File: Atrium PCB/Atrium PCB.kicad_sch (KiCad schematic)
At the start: 495 parts, among them J1 Conn_01x05_Pin, SW1 EC11E09244BS, SW10 SW_Push, SW11 SW_Push, SW13 SW_Push, SW14 SW_Push, SW15 SW_Push, SW16 SW_Push, SW18 SW_Push, SW19 SW_Push, SW2 SKRPACE010, SW20 SW_Push, SW22 SW_Push, SW23 SW_Push, SW24 SW_Push, SW26 SW_Push, SW27 SW_Push, SW28 SW_Push, SW3 SKRPACE010, SW30 SW_Push, SW31 SW_Push, SW32 SW_Push, SW34 SW_Push, SW35 SW_Push, SW36 SW_Push, SW38 SW_Push, SW39 SW_Push, SW4 SW_Push, SW40 SW_Push, SW42 SW_Push, SW43 SW_Push, SW44 SW_Push, SW45 SW_Push, SW46 SW_Push, SW47 SW_Push, SW48 SW_Push, SW49 SW_Push, SW5 SW_Push, SW50 SW_Push, SW51 SW_Push, SW52 SW_Push, SW53 SW_Push, SW54 SW_Push, SW6 SW_Push, SW8 SW_Push, SW9 SW_Push, U12 AP2112K-3.3, U2 LSM6DS3TR-C, U6 SN74LVC1T45DBVR, X1 X322512MSB4SI

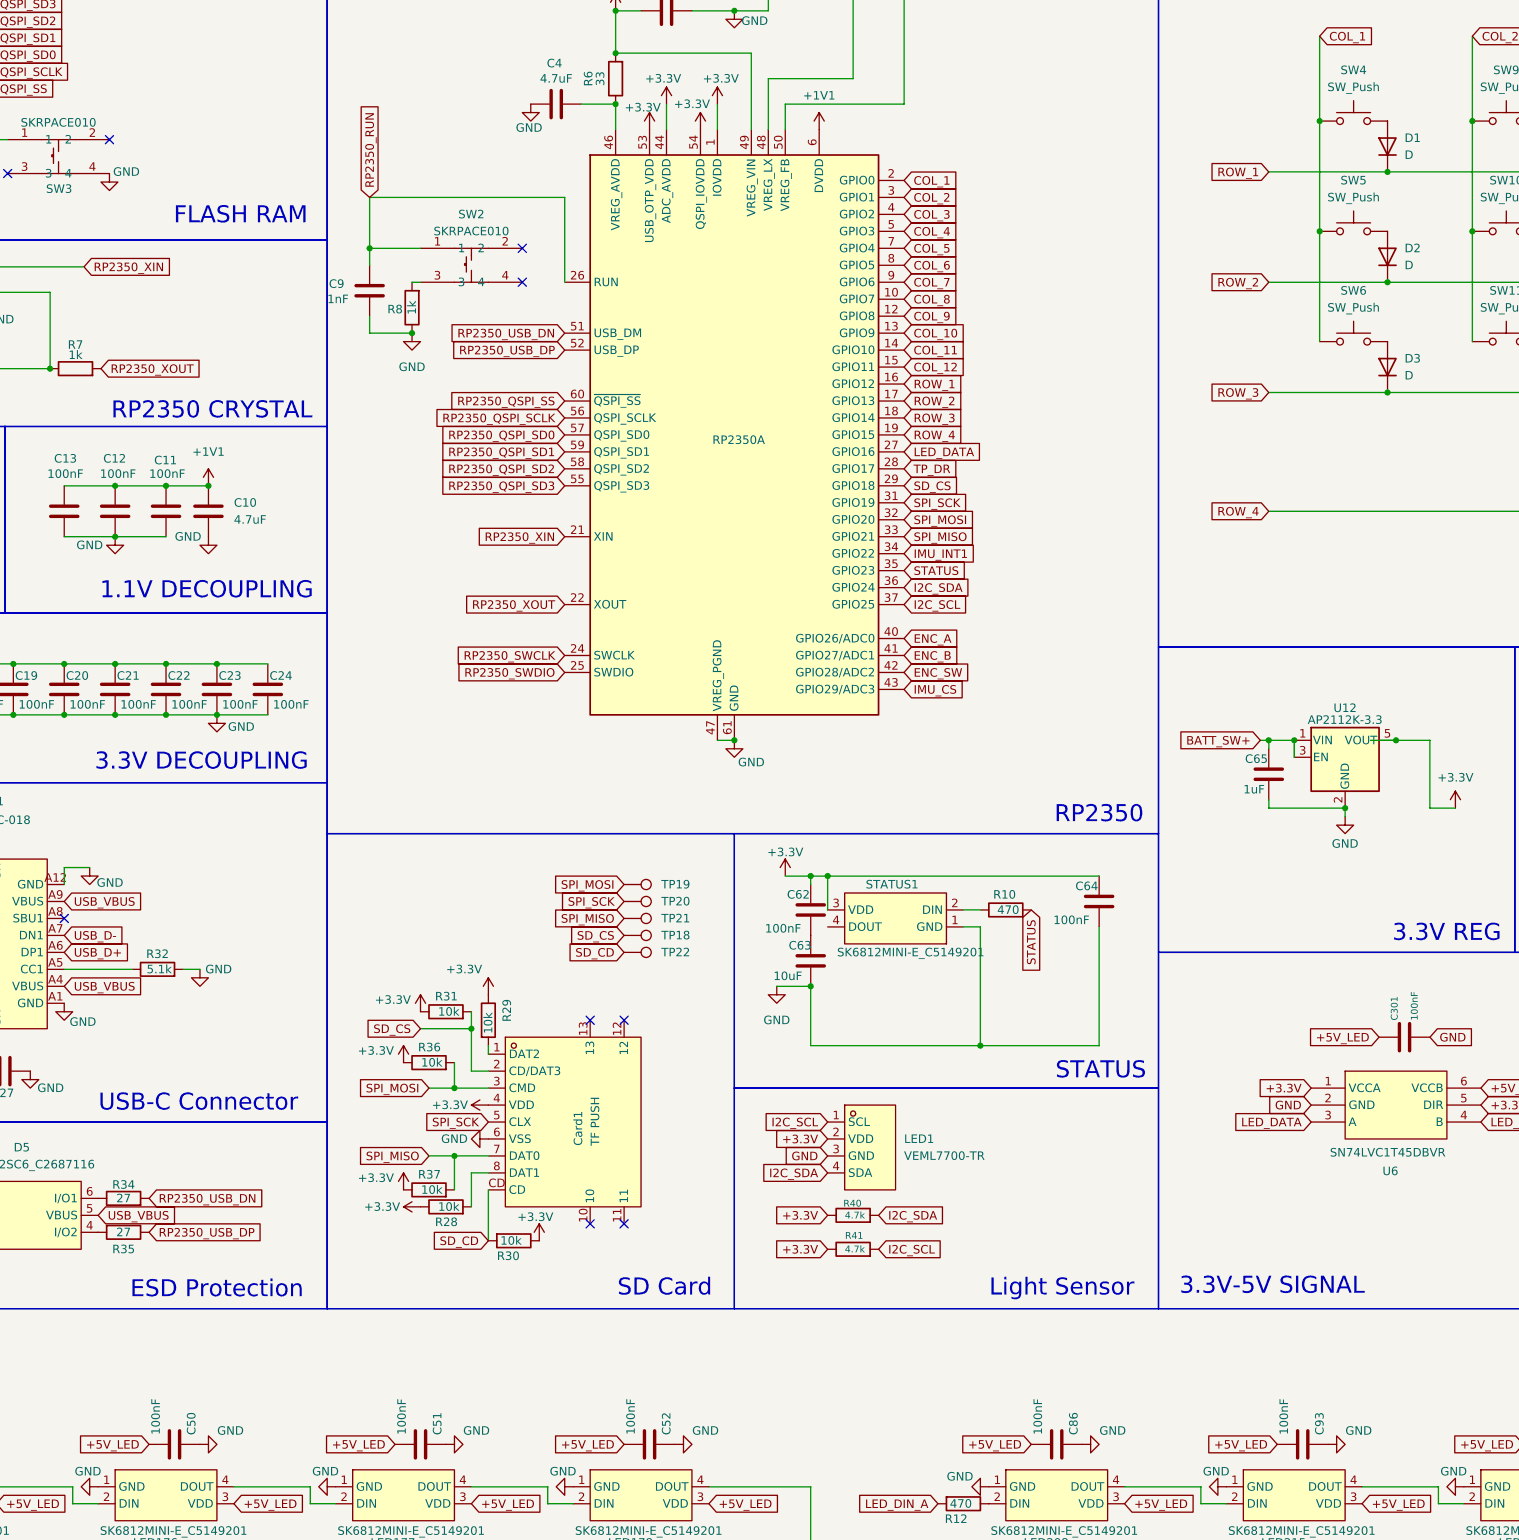
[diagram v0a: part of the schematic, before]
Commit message: sync
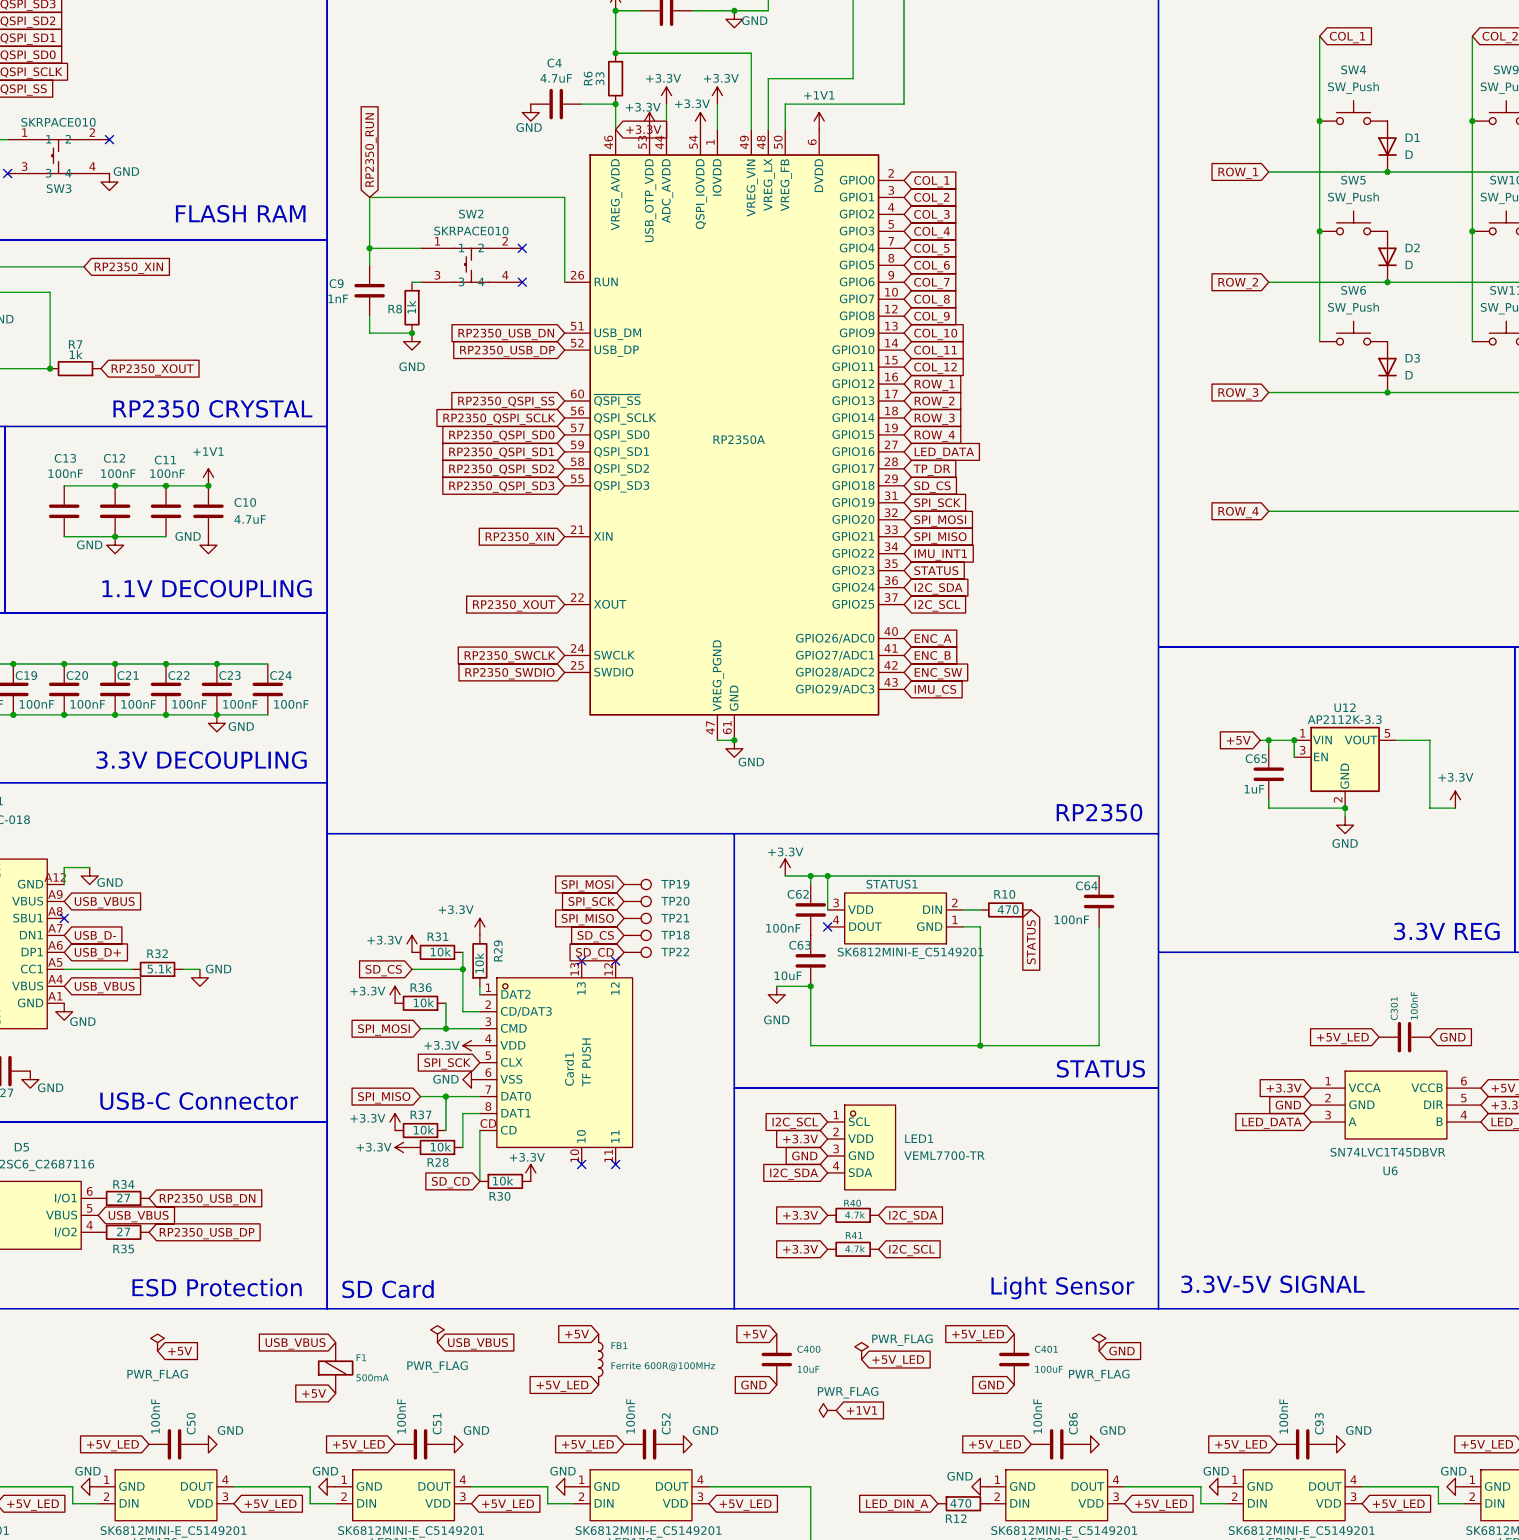
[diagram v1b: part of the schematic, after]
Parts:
- added C400: 10uF, Capacitor_SMD:C_0805_2012Metric, symbol Device:C
- added C401: 100uF, Capacitor_SMD:C_1206_3216Metric, symbol Device:C
- added F1: 500mA, Fuse:Fuse_1206_3216Metric, symbol Device:Polyfuse
- added FB1: Ferrite 600R@100MHz, Inductor_SMD:L_0805_2012Metric, symbol Device:L
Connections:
- net +3.3V: now also C4.2, R6.1, RP2350.46 (VREG_AVDD)
- net +5V_LED: now also C401.1, FB1.2
- net GND: now also C400.2, C401.2
- net USB_VBUS: now also F1.1
- net BATT_SW+ renamed +5V
- net +5V: now also C400.1, F1.2, FB1.1
- no-connect marks 20 -> 21
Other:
- moved on the sheet: Card1, R28, R29, R30, R31, R36, R37
